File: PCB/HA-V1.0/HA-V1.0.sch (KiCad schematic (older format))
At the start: 1 part, among them U1 ATMEGA328P-ANR

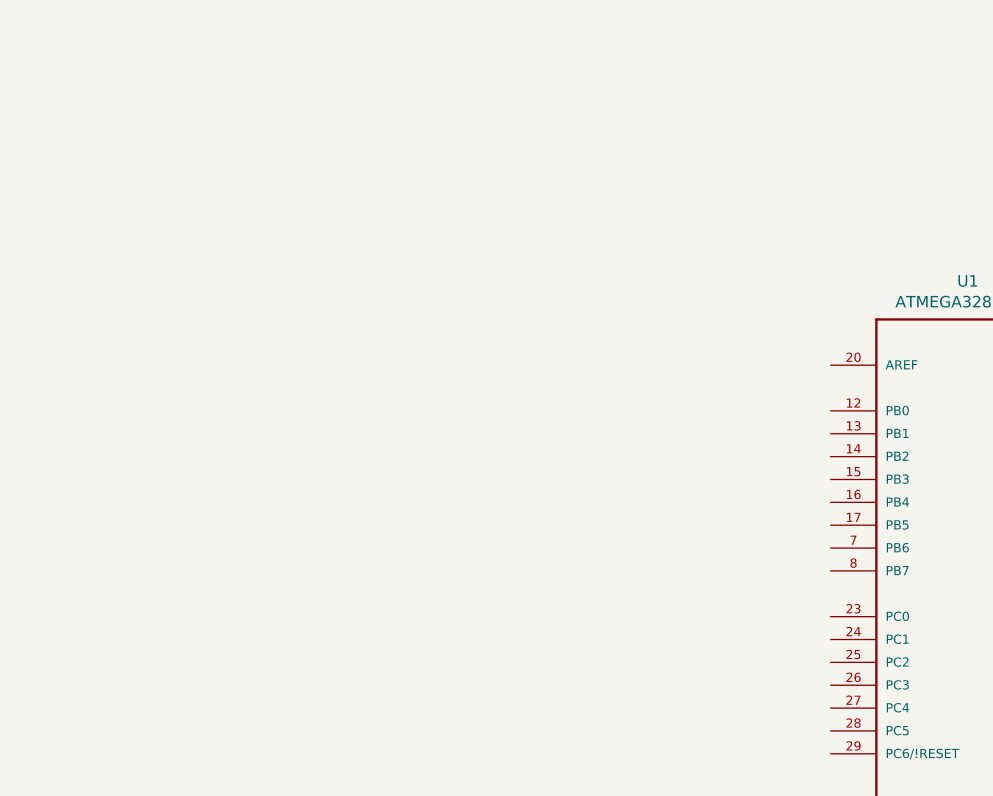
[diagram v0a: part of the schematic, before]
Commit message: Firmware- Scratch
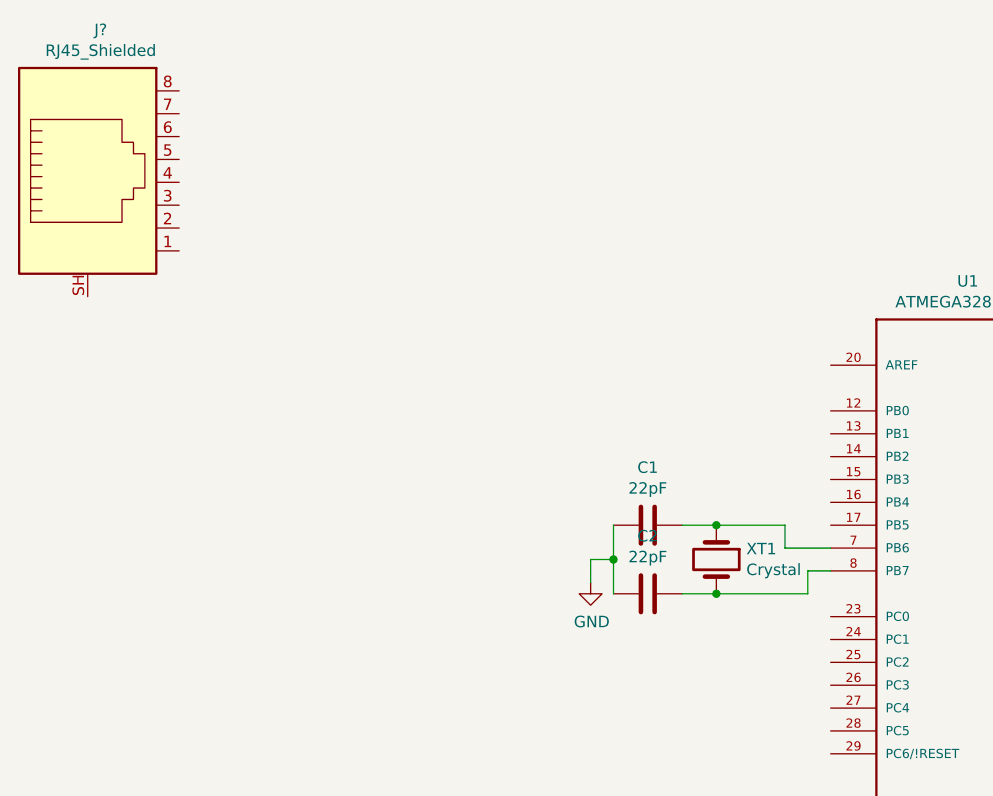
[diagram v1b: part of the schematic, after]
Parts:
- added C1, C2: 22pF, Capacitor_THT:C_Disc_D3.0mm_W1.6mm_P2.50mm, symbol Device:C
- added J?: RJ45_Shielded, symbol Connector:RJ45_Shielded
- added XT1: Crystal, Crystal:Crystal_HC52-U_Vertical, symbol Device:Crystal
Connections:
- net at U1.7 (PB6): now also C1.1, XT1.1
- net at U1.8 (PB7): now also C2.1, XT1.2
- new net GND: C1.2, C2.2
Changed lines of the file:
@@
+	1    0    0    -1
+$EndComp
+$Comp
+L Device:Crystal XT1
+U 1 1 5F0DD00C
+P 4400 3500
+F 0 "XT1" V 4354 3631 50  0000 L CNN
+F 1 "Crystal" V 4445 3631 50  0000 L CNN
+F 2 "Crystal:Crystal_HC52-U_Vertical" H 4400 3500 50  0001 C CNN
+F 3 "~" H 4400 3500 50  0001 C CNN
+	1    4400 3500
+	0    1    1    0
+$EndComp
+Wire Wire Line
+	4900 3450 4700 3450
+Wire Wire Line
+	4700 3450 4700 3350
+Wire Wire Line
+	4700 3350 4400 3350
+Wire Wire Line
+	4900 3550 4800 3550
+Wire Wire Line
+	4800 3550 4800 3650
+Wire Wire Line
+	4800 3650 4400 3650
+$Comp
+L Device:C C1
+U 1 1 5F0DE508
+P 4100 3350
+F 0 "C1" V 3848 3350 50  0000 C CNN
+F 1 "22pF" V 3939 3350 50  0000 C CNN
+F 2 "Capacitor_THT:C_Disc_D3.0mm_W1.6mm_P2.50mm" H 4138 3200 50  0001 C CNN
+F 3 "~" H 4100 3350 50  0001 C CNN
+	1    4100 3350
+	0    1    1    0
+$EndComp
+$Comp
+L Device:C C2
+U 1 1 5F0DECE8
+P 4100 3650
+F 0 "C2" V 3848 3650 50  0000 C CNN
+F 1 "22pF" V 3939 3650 50  0000 C CNN
+F 2 "Capacitor_THT:C_Disc_D3.0mm_W1.6mm_P2.50mm" H 4138 3500 50  0001 C CNN
+F 3 "~" H 4100 3650 50  0001 C CNN
+	1    4100 3650
+	0    1    1    0
+$EndComp
+Wire Wire Line
+	4250 3350 4400 3350
+Connection ~ 4400 3350
+Wire Wire Line
+	4250 3650 4400 3650
+Connection ~ 4400 3650
+Wire Wire Line
+	3950 3500 3950 3650
+Wire Wire Line
+	3950 3350 3950 3500
+Connection ~ 3950 3500
+Wire Wire Line
+	3850 3500 3950 3500
+Wire Wire Line
+	3850 3600 3850 3500
+$Comp
+L power:GND #PWR0101
+U 1 1 5F0DF791
+P 3850 3600
+F 0 "#PWR0101" H 3850 3350 50  0001 C CNN
+F 1 "GND" H 3855 3427 50  0000 C CNN
+F 2 "" H 3850 3600 50  0001 C CNN
+F 3 "" H 3850 3600 50  0001 C CNN
+	1    3850 3600
+	1    0    0    -1
+$EndComp
+$Comp
+L Connector:RJ45_Shielded J?
+U 1 1 5F0DEB93
+P 1650 1850
+F 0 "J?" H 1707 2517 50  0000 C CNN
+F 1 "RJ45_Shielded" H 1707 2426 50  0000 C CNN
+F 2 "" V 1650 1875 50  0001 C CNN
+F 3 "~" V 1650 1875 50  0001 C CNN
+	1    1650 1850
 	1    0    0    -1
 $EndComp

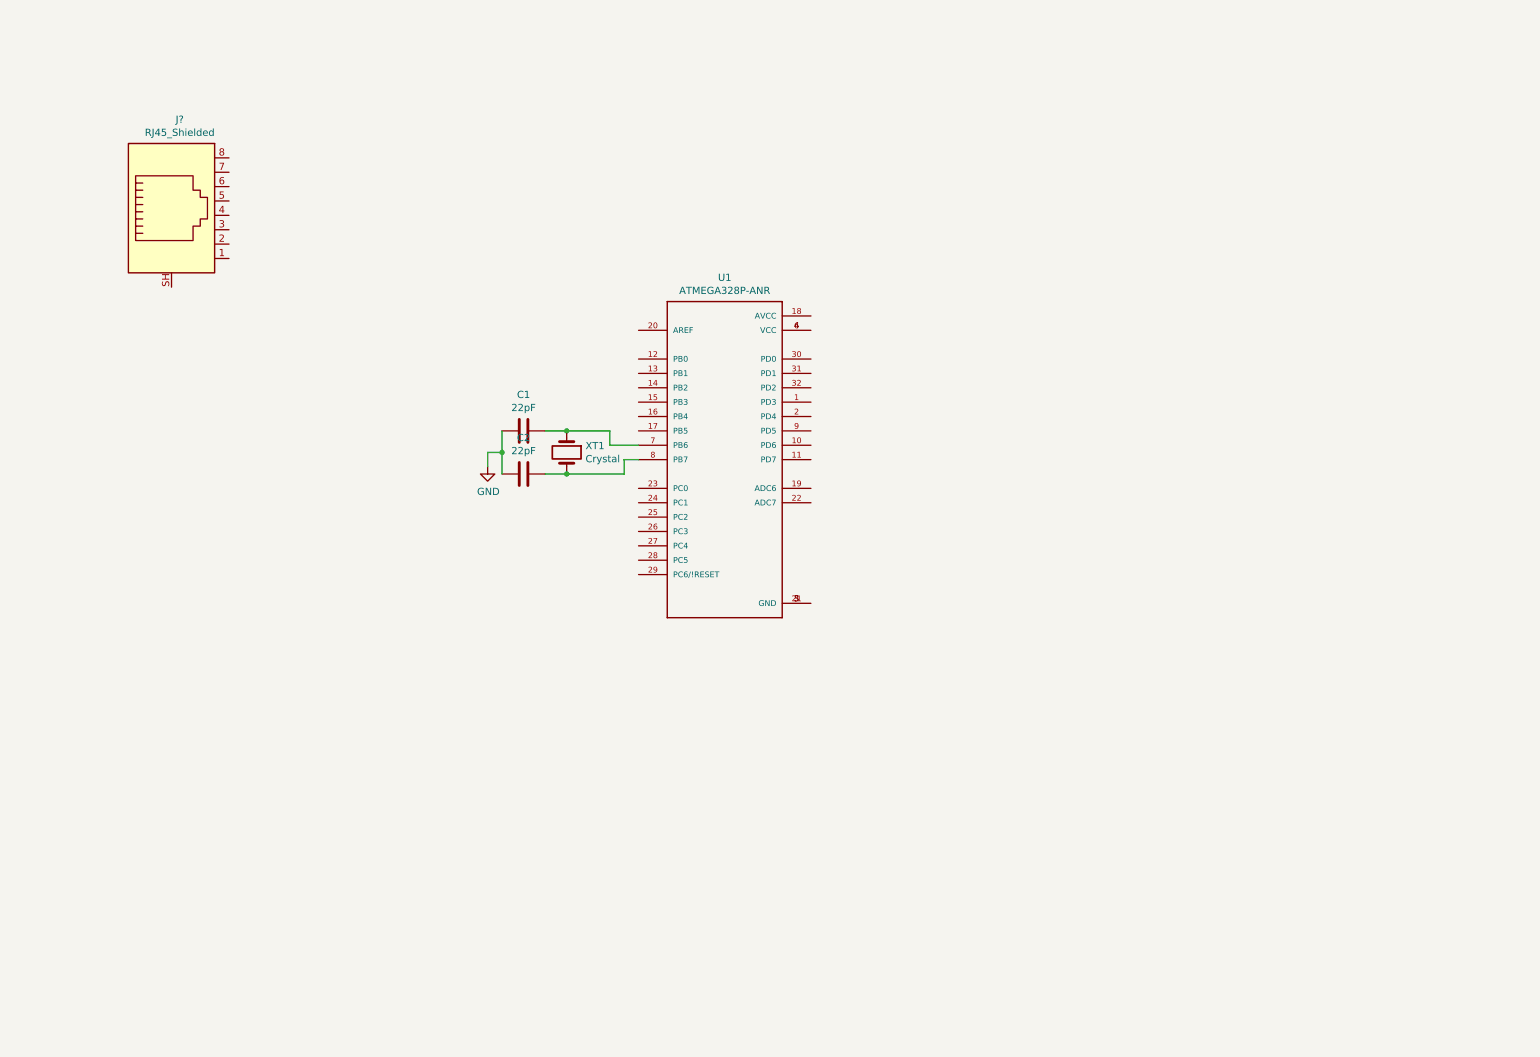
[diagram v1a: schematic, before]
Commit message: Delete ATSD PROJ
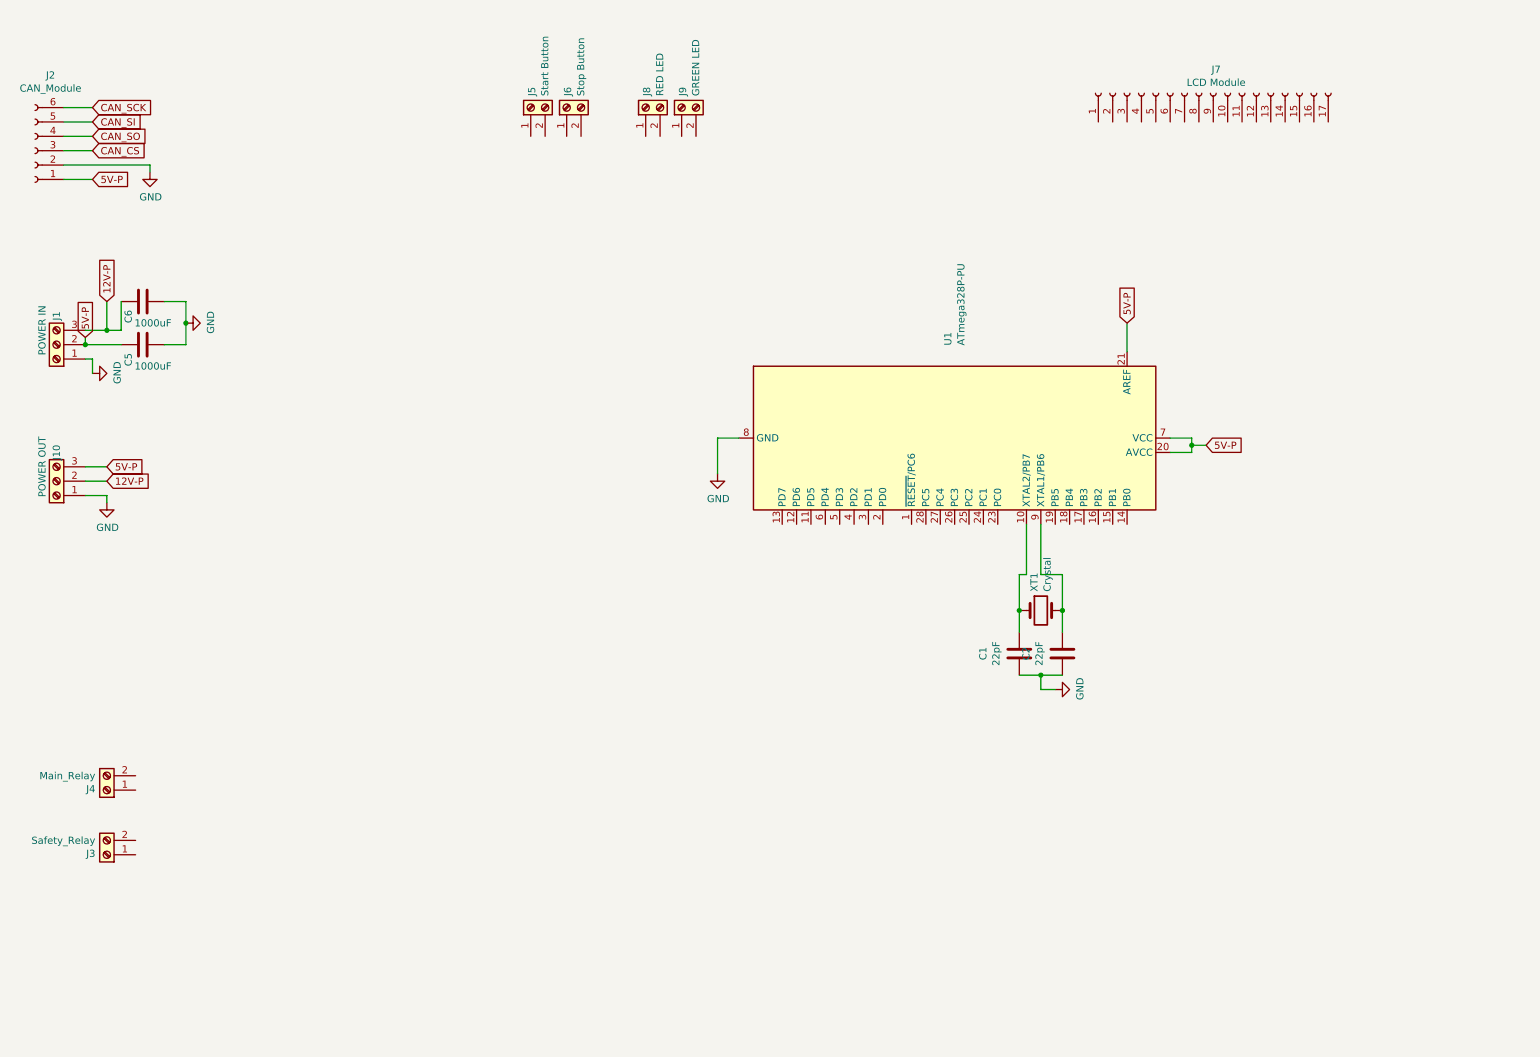
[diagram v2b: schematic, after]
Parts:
- removed J?: RJ45_Shielded, symbol Connector:RJ45_Shielded
- removed U1: ATMEGA328P-ANR, Package_QFP:QFP80P900X900X120-32N, symbol ATMEGA328P-ANR:ATMEGA328P-ANR
- added C5, C6: 1000uF, Capacitor_THT:CP_Radial_D10.0mm_P5.00mm, symbol Device:C
- added J1: POWER IN, Connector_TE-Connectivity:TE_826576-3_1x03_P3.96mm_Vertical, symbol Connector:Screw_Terminal_01x03
- added J10: POWER OUT, Connector_TE-Connectivity:TE_826576-3_1x03_P3.96mm_Vertical, symbol Connector:Screw_Terminal_01x03
- added J2: CAN_Module, Connector_PinHeader_2.54mm:PinHeader_1x06_P2.54mm_Vertical, symbol Connector:Conn_01x06_Female
- added J3: Safety_Relay, Connector_TE-Connectivity:TE_826576-2_1x02_P3.96mm_Vertical, symbol Connector:Screw_Terminal_01x02
- added J4: Main_Relay, Connector_TE-Connectivity:TE_826576-2_1x02_P3.96mm_Vertical, symbol Connector:Screw_Terminal_01x02
- added J5: Start Button, Connector_TE-Connectivity:TE_826576-2_1x02_P3.96mm_Vertical, symbol Connector:Screw_Terminal_01x02
- added J6: Stop Button, Connector_TE-Connectivity:TE_826576-2_1x02_P3.96mm_Vertical, symbol Connector:Screw_Terminal_01x02
- added J7: LCD Module, Connector_PinHeader_2.54mm:PinHeader_1x16_P2.54mm_Vertical, symbol Connector:Conn_01x17_Female
- added J8: RED LED, Connector_TE-Connectivity:TE_826576-2_1x02_P3.96mm_Vertical, symbol Connector:Screw_Terminal_01x02
- added J9: GREEN LED, Connector_TE-Connectivity:TE_826576-2_1x02_P3.96mm_Vertical, symbol Connector:Screw_Terminal_01x02
- added U1: ATmega328P-PU, Package_DIP:DIP-28_W7.62mm, symbol MCU_Microchip_ATmega:ATmega328P-PU
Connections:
- net GND: now also C5.2, C6.2, J1.1 (Pin_1), J10.1 (Pin_1), J2.2 (Pin_2), U1.22 (GND), U1.8 (GND)
- net at C1.1, XT1.1: now also U1.10 (XTAL2/PB7)
- net at C2.1, XT1.2: now also U1.9 (XTAL1/PB6)
- new net 12V-P: C6.1, J1.3 (Pin_3), J10.2 (Pin_2)
- new net 5V-P: C5.1, J1.2 (Pin_2), J10.3 (Pin_3), J2.1 (Pin_1), U1.20 (AVCC), U1.21 (AREF), U1.7 (VCC)
- new net CAN_CS: J2.3 (Pin_3)
- new net CAN_SCK: J2.6 (Pin_6)
- new net CAN_SI: J2.5 (Pin_5)
- new net CAN_SO: J2.4 (Pin_4)
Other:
- moved on the sheet: C1, C2, XT1

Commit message: Final PCB Fabrication Done
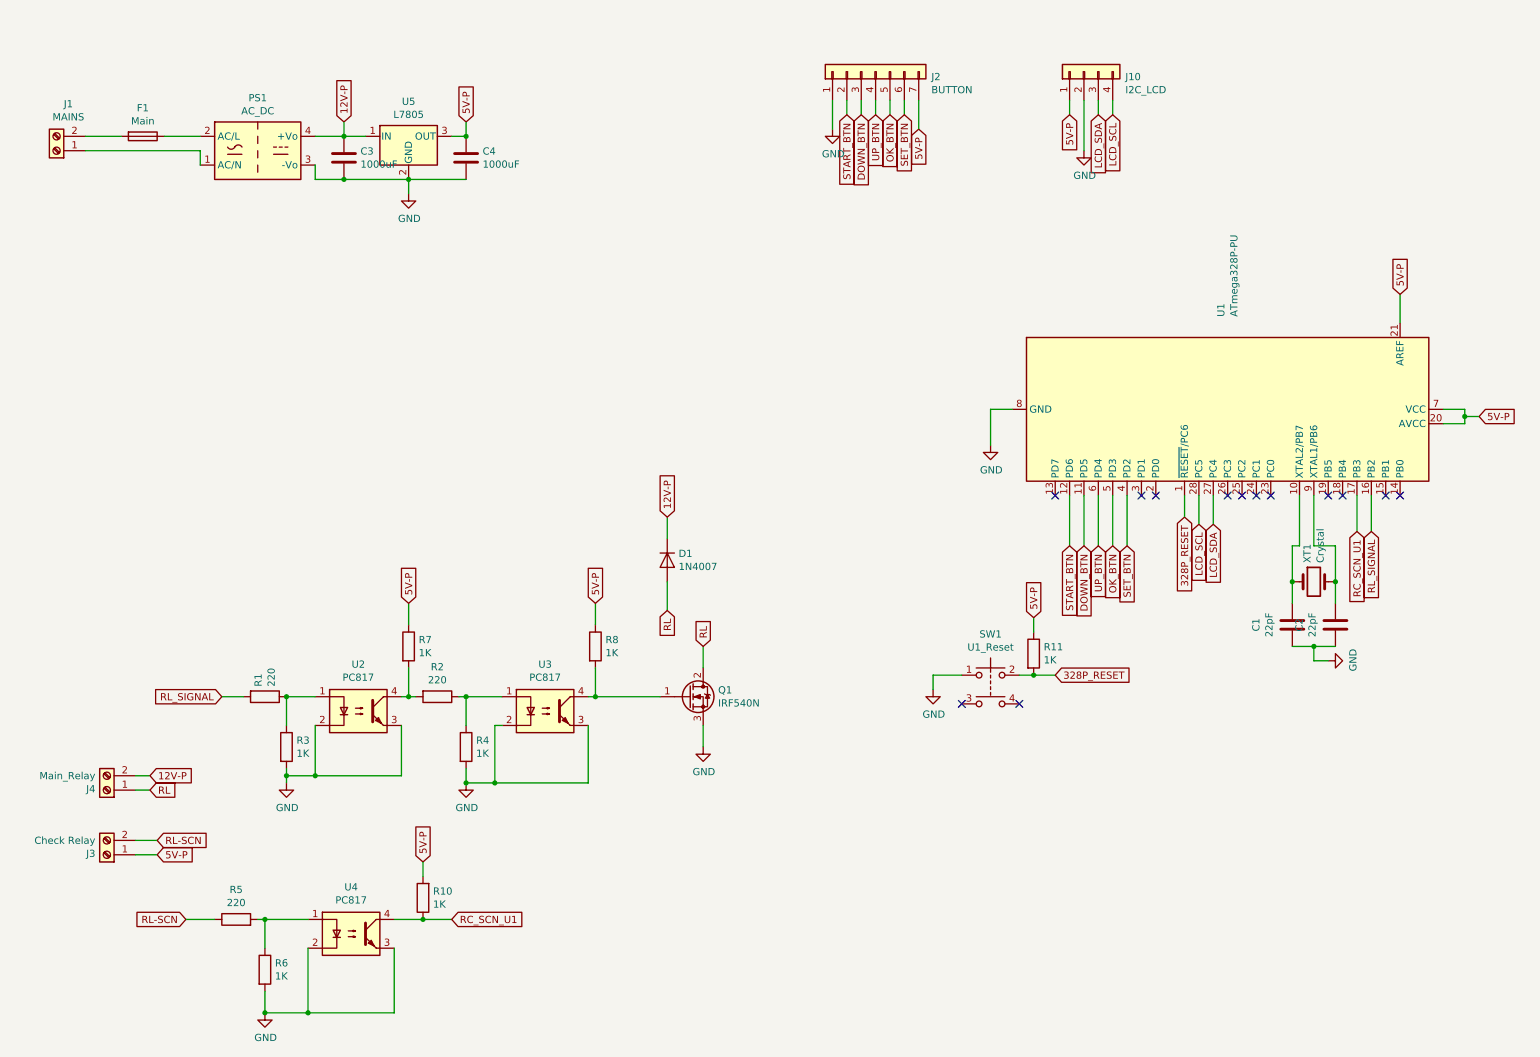
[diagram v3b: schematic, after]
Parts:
- removed C5, C6: 1000uF, Capacitor_THT:CP_Radial_D10.0mm_P5.00mm, symbol Device:C
- removed J1: POWER IN, Connector_TE-Connectivity:TE_826576-3_1x03_P3.96mm_Vertical, symbol Connector:Screw_Terminal_01x03
- removed J10: POWER OUT, Connector_TE-Connectivity:TE_826576-3_1x03_P3.96mm_Vertical, symbol Connector:Screw_Terminal_01x03
- removed J2: CAN_Module, Connector_PinHeader_2.54mm:PinHeader_1x06_P2.54mm_Vertical, symbol Connector:Conn_01x06_Female
- removed J5: Start Button, Connector_TE-Connectivity:TE_826576-2_1x02_P3.96mm_Vertical, symbol Connector:Screw_Terminal_01x02
- removed J6: Stop Button, Connector_TE-Connectivity:TE_826576-2_1x02_P3.96mm_Vertical, symbol Connector:Screw_Terminal_01x02
- removed J7: LCD Module, Connector_PinHeader_2.54mm:PinHeader_1x16_P2.54mm_Vertical, symbol Connector:Conn_01x17_Female
- removed J8: RED LED, Connector_TE-Connectivity:TE_826576-2_1x02_P3.96mm_Vertical, symbol Connector:Screw_Terminal_01x02
- removed J9: GREEN LED, Connector_TE-Connectivity:TE_826576-2_1x02_P3.96mm_Vertical, symbol Connector:Screw_Terminal_01x02
- added C3, C4: 1000uF, Capacitor_THT:C_Radial_D10.0mm_H16.0mm_P5.00mm, symbol Device:C
- added D1: 1N4007, Diode_THT:D_DO-41_SOD81_P10.16mm_Horizontal, symbol Diode:1N4007
- added F1: Main, Fuse:Fuse_SunFuse-6HP, symbol Device:Fuse
- added J1: MAINS, Connector_Phoenix_MC_HighVoltage:PhoenixContact_MCV_1,5_2-G-5.08_1x02_P5.08mm_Vertical, symbol Connector:Screw_Terminal_01x02
- added J10: I2C_LCD, Connector_PinHeader_2.54mm:PinHeader_1x04_P2.54mm_Vertical, symbol Connector_Generic:Conn_01x04
- added J2: BUTTON, Connector_PinSocket_2.54mm:PinSocket_1x07_P2.54mm_Vertical, symbol Connector_Generic:Conn_01x07
- added PS1: AC_DC, Converter_ACDC:Converter_ACDC_MeanWell_IRM-10-xx_THT, symbol Converter_ACDC:IRM-10-12
- added Q1: IRF540N, Package_TO_SOT_THT:TO-220-3_Vertical, symbol Transistor_FET:IRF540N
- added R1, R2, R5: 220, Resistor_THT:R_Axial_DIN0207_L6.3mm_D2.5mm_P7.62mm_Horizontal, symbol Device:R
- added R10, R11, R3, R4, R6, R7, R8: 1K, Resistor_THT:R_Axial_DIN0207_L6.3mm_D2.5mm_P7.62mm_Horizontal, symbol Device:R
- added SW1: U1_Reset, Button_Switch_THT:SW_PUSH_6mm_H4.3mm, symbol Switch:SW_Push_Dual
- added U2, U3, U4: PC817, Package_DIP:DIP-4_W7.62mm, symbol Isolator:PC817
- added U5: L7805, Package_TO_SOT_THT:TO-220-3_Vertical, symbol Regulator_Linear:L7805
- J3: value Safety_Relay -> Check Relay
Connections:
- net 12V-P: now also J4.2 (Pin_2), C3.1, D1.1 (K), PS1.4 (+Vo), U5.1 (IN)
- net 5V-P: now also J3.1 (Pin_1), C4.1, J10.1 (Pin_1), J2.7 (Pin_7), R10.2, R11.1, R7.1, R8.1, U5.3 (OUT)
- net GND: now also C3.2, C4.2, J10.2 (Pin_2), J2.1 (Pin_1), PS1.3 (-Vo), Q1.3 (S), R3.2, R4.2, R6.2, SW1.1, U2.2, U2.3, U3.2, U3.3, U4.2, U4.3, U5.2 (GND)
- net RL-SCN: now reaches J3.2 (Pin_2)
- net RL-SCN: now also R5.1
- net RL: now reaches J4.1 (Pin_1)
- net RL: now also D1.2 (A), Q1.2 (D)
- net 328P_RESET: now reaches U1.1 (~RESET~/PC6)
- net 328P_RESET: now also R11.2, SW1.2
- net DOWN_BTN: now reaches U1.11 (PD5)
- net DOWN_BTN: now also J2.3 (Pin_3)
- net START_BTN: now reaches U1.12 (PD6)
- net START_BTN: now also J2.2 (Pin_2)
- net RL_SIGNAL: now reaches U1.16 (PB2)
- net RL_SIGNAL: now also R1.2
- net RC_SCN_U1: now reaches U1.17 (PB3)
- net RC_SCN_U1: now also R10.1, U4.4
- net LCD_SDA: now reaches U1.27 (PC4)
- net LCD_SDA: now also J10.3 (Pin_3)
- net LCD_SCL: now reaches U1.28 (PC5)
- net LCD_SCL: now also J10.4 (Pin_4)
- net SET_BTN: now reaches U1.4 (PD2)
- net SET_BTN: now also J2.6 (Pin_6)
- net OK_BTN: now reaches U1.5 (PD3)
- net OK_BTN: now also J2.5 (Pin_5)
- net UP_BTN: now reaches U1.6 (PD4)
- net UP_BTN: now also J2.4 (Pin_4)
- new net: R1.1, R3.1, U2.1
- new net: R2.2, R7.2, U2.4
- new net: R2.1, R4.1, U3.1
- new net: Q1.1 (G), R8.2, U3.4
- new net: R5.2, R6.1, U4.1
- new net: J1.1 (Pin_1), PS1.1 (AC/N)
- new net: F1.1, PS1.2 (AC/L)
- new net: F1.2, J1.2 (Pin_2)
- no-connect marks 0 -> 13
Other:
- moved on the sheet: C1, C2, U1, XT1
